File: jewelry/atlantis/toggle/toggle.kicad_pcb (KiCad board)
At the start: 2 copper layers, 24 x 24 mm, 11 parts, among them Q1 Q_PMOS_DGS, U1 74LVC2G04

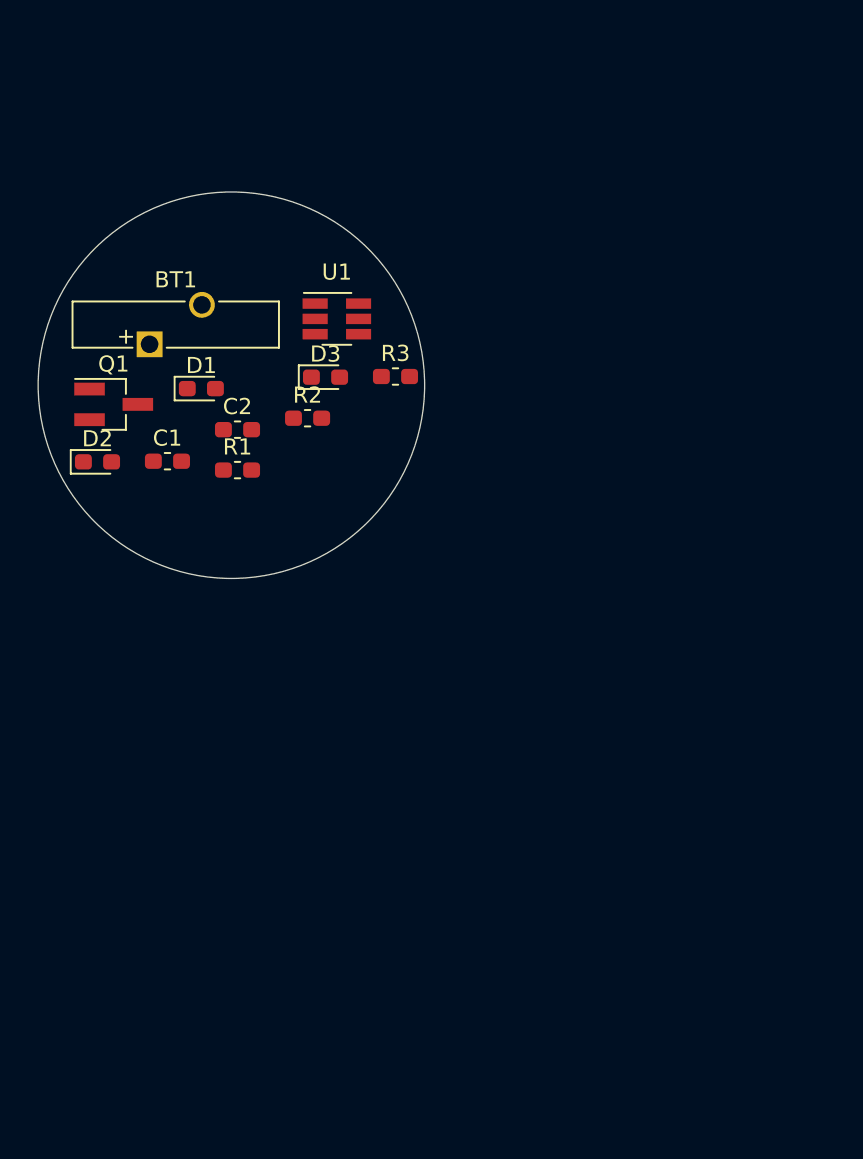
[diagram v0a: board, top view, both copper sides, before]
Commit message: atlantis: Rough PCB for earthing
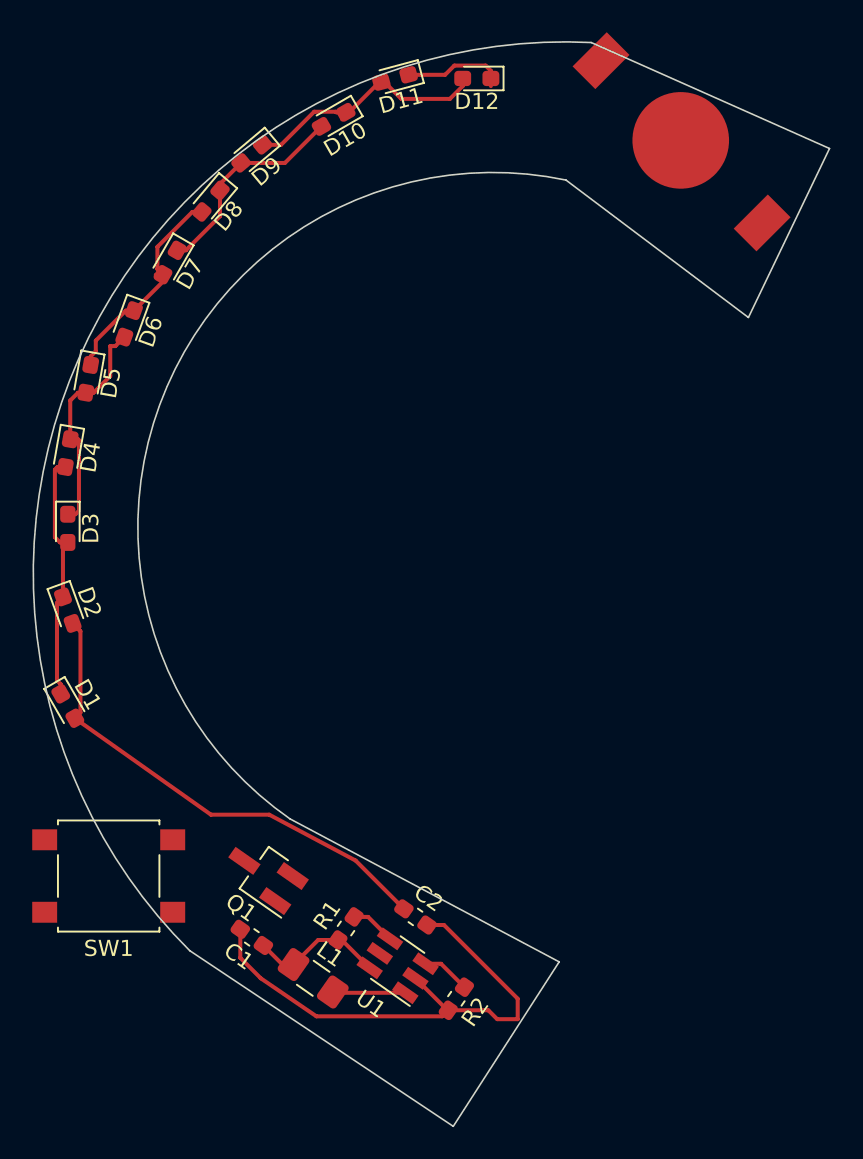
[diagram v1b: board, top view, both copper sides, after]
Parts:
- removed R3: R, Resistor_SMD:R_0603_1608Metric_Pad1.05x0.95mm_HandSolder
- added D10: LED, LED_SMD:LED_0603_1608Metric_Pad1.05x0.95mm_HandSolder, F.Cu at (94.0, 64.8)
- added D11: LED, LED_SMD:LED_0603_1608Metric_Pad1.05x0.95mm_HandSolder, F.Cu at (97.8, 62.2)
- added D12: LED, LED_SMD:LED_0603_1608Metric_Pad1.05x0.95mm_HandSolder, F.Cu at (102.9, 62.2)
- added D4: LED, LED_SMD:LED_0603_1608Metric_Pad1.05x0.95mm_HandSolder, F.Cu at (77.5, 85.5)
- added D5: LED, LED_SMD:LED_0603_1608Metric_Pad1.05x0.95mm_HandSolder, F.Cu at (78.7, 80.9)
- added D6: LED, LED_SMD:LED_0603_1608Metric_Pad1.05x0.95mm_HandSolder, F.Cu at (81.3, 77.5)
- added D7: LED, LED_SMD:LED_0603_1608Metric_Pad1.05x0.95mm_HandSolder, F.Cu at (83.8, 73.7)
- added D8: LED, LED_SMD:LED_0603_1608Metric_Pad1.05x0.95mm_HandSolder, F.Cu at (86.4, 69.8)
- added D9: LED, LED_SMD:LED_0603_1608Metric_Pad1.05x0.95mm_HandSolder, F.Cu at (88.9, 66.9)
- added L1: L, Inductor_SMD:L_1206_3216Metric_Pad1.42x1.75mm_HandSolder, F.Cu at (92.7, 118.1)
- added SW1: SW_SPST, Button_Switch_SMD:SW_SPST_B3S-1000, F.Cu at (80.0, 111.8)
- BT1: value Battery_Cell -> CR1216; footprint Battery:Battery_Panasonic_CR1220-VCN_Vertical_CircularHoles -> touchled:Battery_CR1225
- C1: value 1nF -> 1uF
- C2: value 100nF -> 1uF
- Q1: value Q_PMOS_DGS -> BSS138L
- R1: value 10k -> 100k
- R2: value 100k -> 220R
- U1: value 74LVC2G04 -> AP3019A; footprint Package_TO_SOT_SMD:SOT-23-6_Handsoldering -> touchled:SOT-223-6-extraspace
- moved U1 40.4 mm to (98.0, 117.3), turned to 145 degrees
- moved R2 37.2 mm to (101.6, 119.4), turned to 235 degrees
- moved BT1 35.4 mm to (115.6, 66.0), turned to 315 degrees
- moved C2 32.2 mm to (99.1, 114.3), turned to 325 degrees
- moved Q1 30.7 mm to (89.7, 111.7), turned to 145 degrees
- moved C1 30.0 mm to (88.9, 115.6), turned to 145 degrees
- moved R1 29.3 mm to (94.7, 115.0), turned to 55 degrees
- moved D1 21.4 mm to (77.5, 101.2), turned to 300 degrees
- moved D3 18.6 mm to (77.5, 90.2), turned to 270 degrees
- moved D2 9.39 mm to (77.5, 95.2), turned to 290 degrees
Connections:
- BT1 pad 2: GND -> Net-(BT1-Pad2)
- C1 pad 1: Net-(C1-Pad1) -> VCC
- C2 pad 1: Net-(C2-Pad1) -> /LED+
- D1 pad 1: GND -> Net-(D1-Pad1)
- D1 pad 2: Net-(D1-Pad2) -> /LED+
- D2 pad 1: GND -> Net-(D1-Pad1)
- D2 pad 2: Net-(D1-Pad2) -> /LED+
- D3 pad 1: GND -> Net-(D3-Pad1)
- D3 pad 2: Net-(D1-Pad2) -> Net-(D1-Pad1)
- Q1 pad 1: Net-(BT1-Pad1) -> GND
- Q1 pad 2: GND -> Net-(BT1-Pad2)
- Q1 pad 3: VCC -> Net-(BT1-Pad1)
- R1 pad 1: /OUT -> VCC
- R1 pad 2: Net-(C1-Pad1) -> Net-(R1-Pad2)
- R2 pad 1: Net-(R2-Pad1) -> /LED-
- R2 pad 2: Net-(C2-Pad1) -> GND
- U1 pad 1: Net-(C1-Pad1) -> Net-(L1-Pad2)
- U1 pad 3: Net-(R2-Pad1) -> /LED-
- U1 pad 4: /OUT -> Net-(R1-Pad2)
- U1 pad 5: VCC -> /LED+
- U1 pad 6: Net-(R2-Pad1) -> VCC
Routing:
- net GND: track 0.00 -> 32.3 mm
- net /LED+: track 0.00 -> 30.5 mm
- net Net-(D1-Pad1): track 0.00 -> 15.6 mm
- net Net-(D10-Pad1): track 0.00 -> 15.6 mm
- net Net-(D3-Pad1): track 0.00 -> 14.2 mm
- net Net-(D5-Pad1): track 0.00 -> 13.7 mm
- net Net-(D10-Pad2): track 0.00 -> 13.3 mm
- net VCC: track 0.00 -> 8.44 mm
- net Net-(D11-Pad1): track 0.00 -> 6.43 mm
- net Net-(L1-Pad2): track 0.00 -> 4.52 mm
- net /LED-: track 0.00 -> 3.01 mm
- net Net-(R1-Pad2): track 0.00 -> 2.79 mm
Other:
- board size 24 x 24 mm -> 49.4 x 67.3 mm
